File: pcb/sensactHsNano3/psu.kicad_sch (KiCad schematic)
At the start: 10 parts, among them U7 RY8310

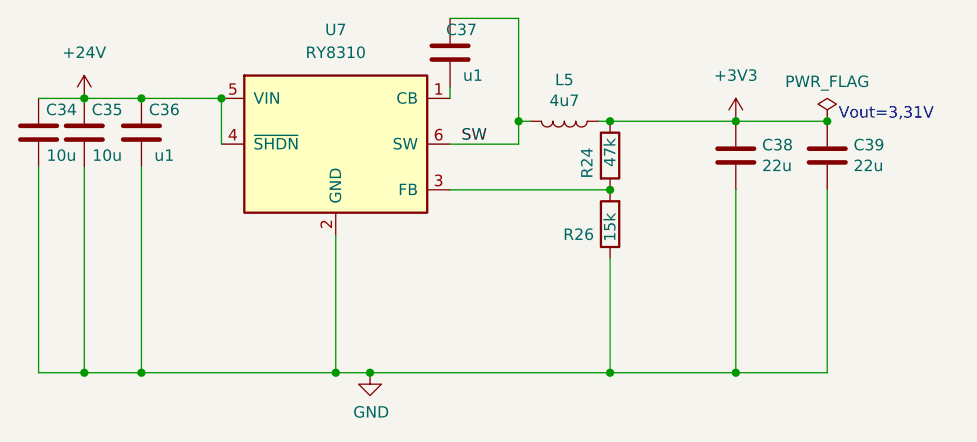
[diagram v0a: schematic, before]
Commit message: Various updates, new version with ESP32 in beta test :-)
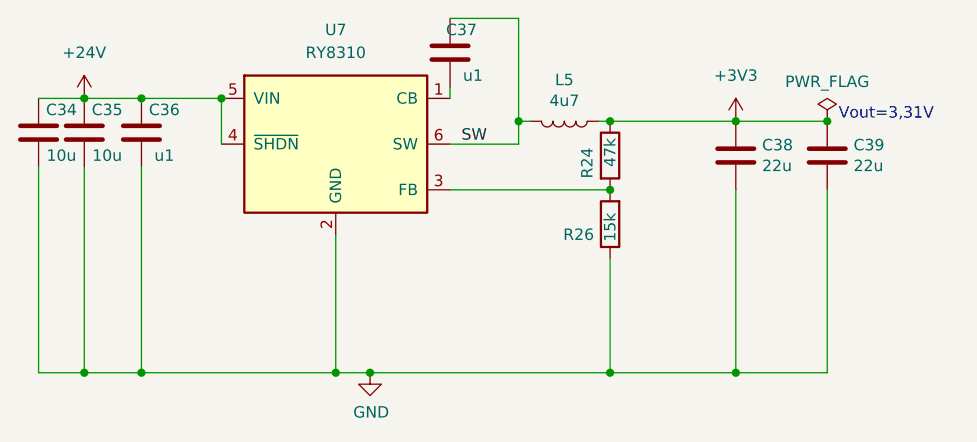
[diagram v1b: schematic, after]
